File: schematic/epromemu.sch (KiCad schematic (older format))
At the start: 6 parts, among them J1 EPROM Connector, U1 Teensy4.1, U2 TXS0108EPW, U3 TXS0108EPW, U4 TXS0108EPW, U5 TXS0108EPW

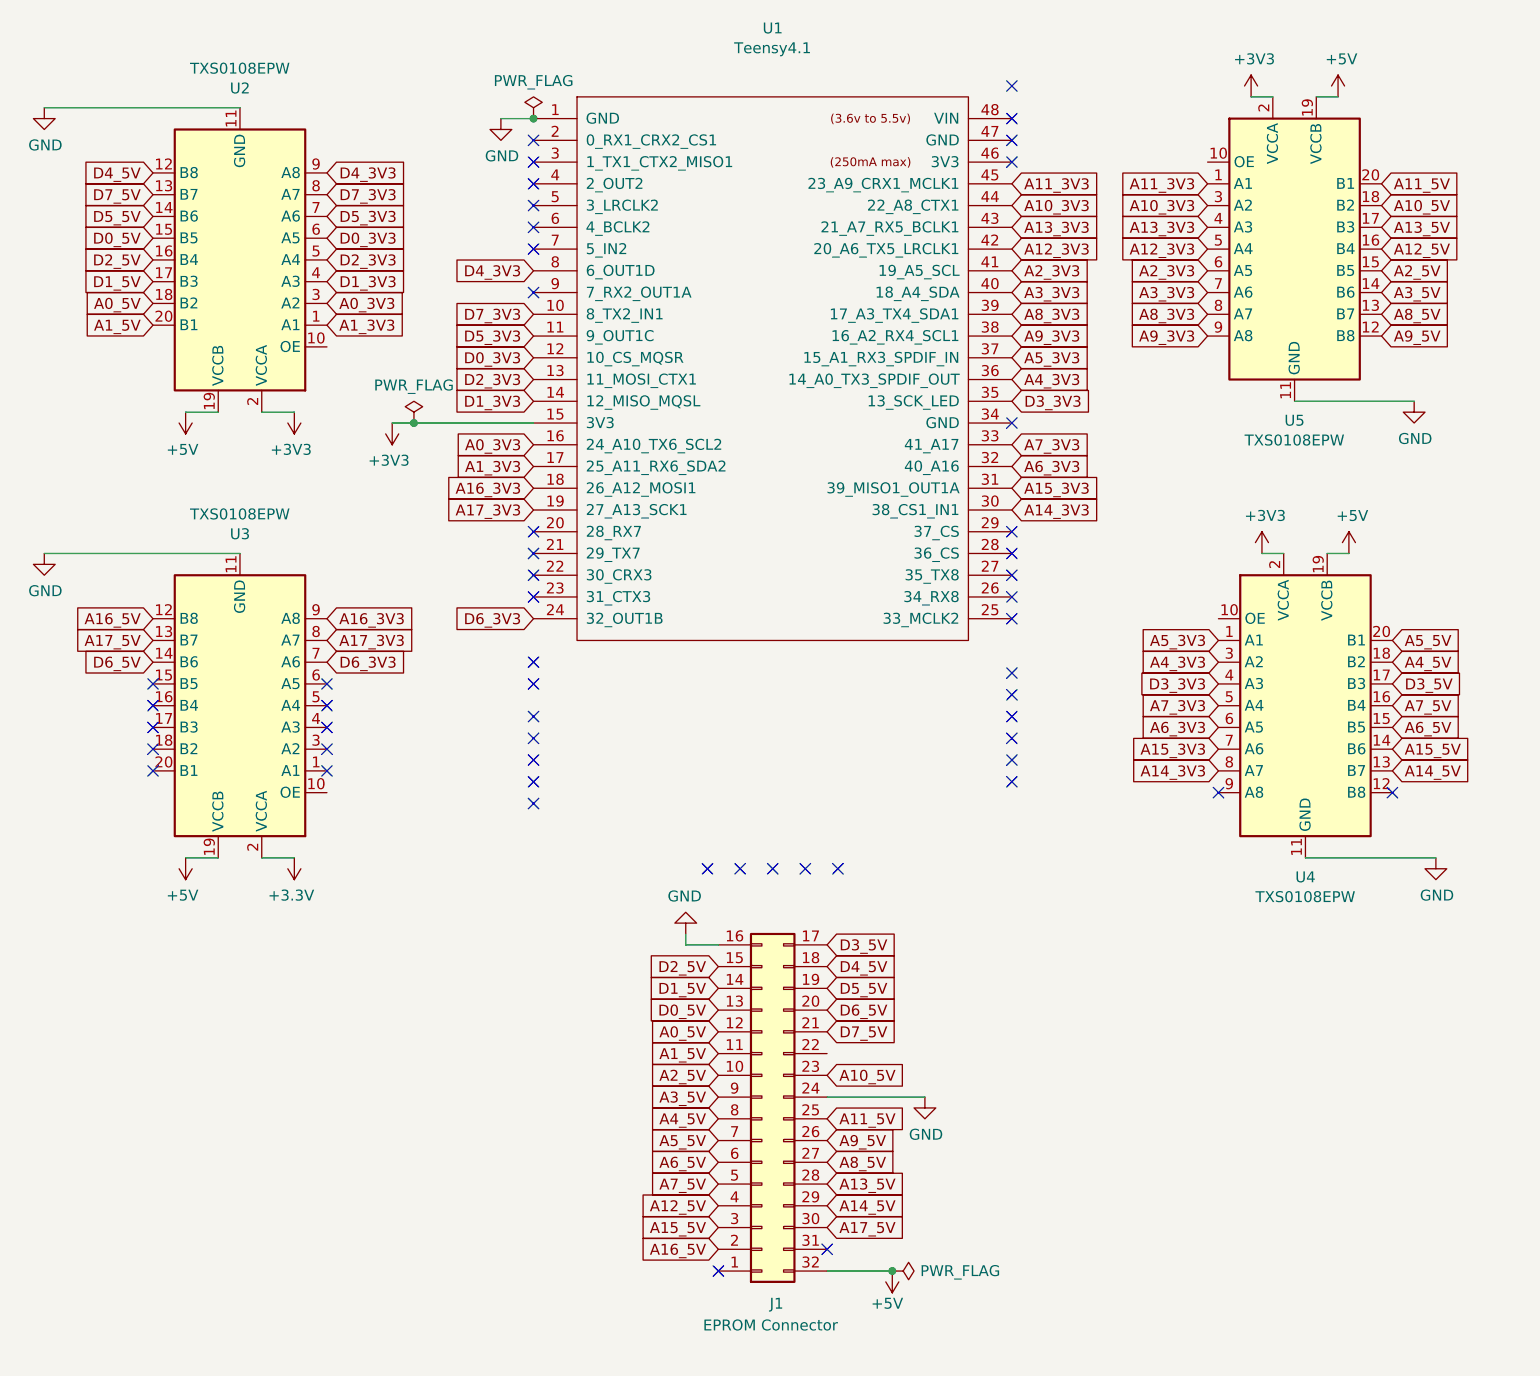
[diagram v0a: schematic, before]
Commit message: updates
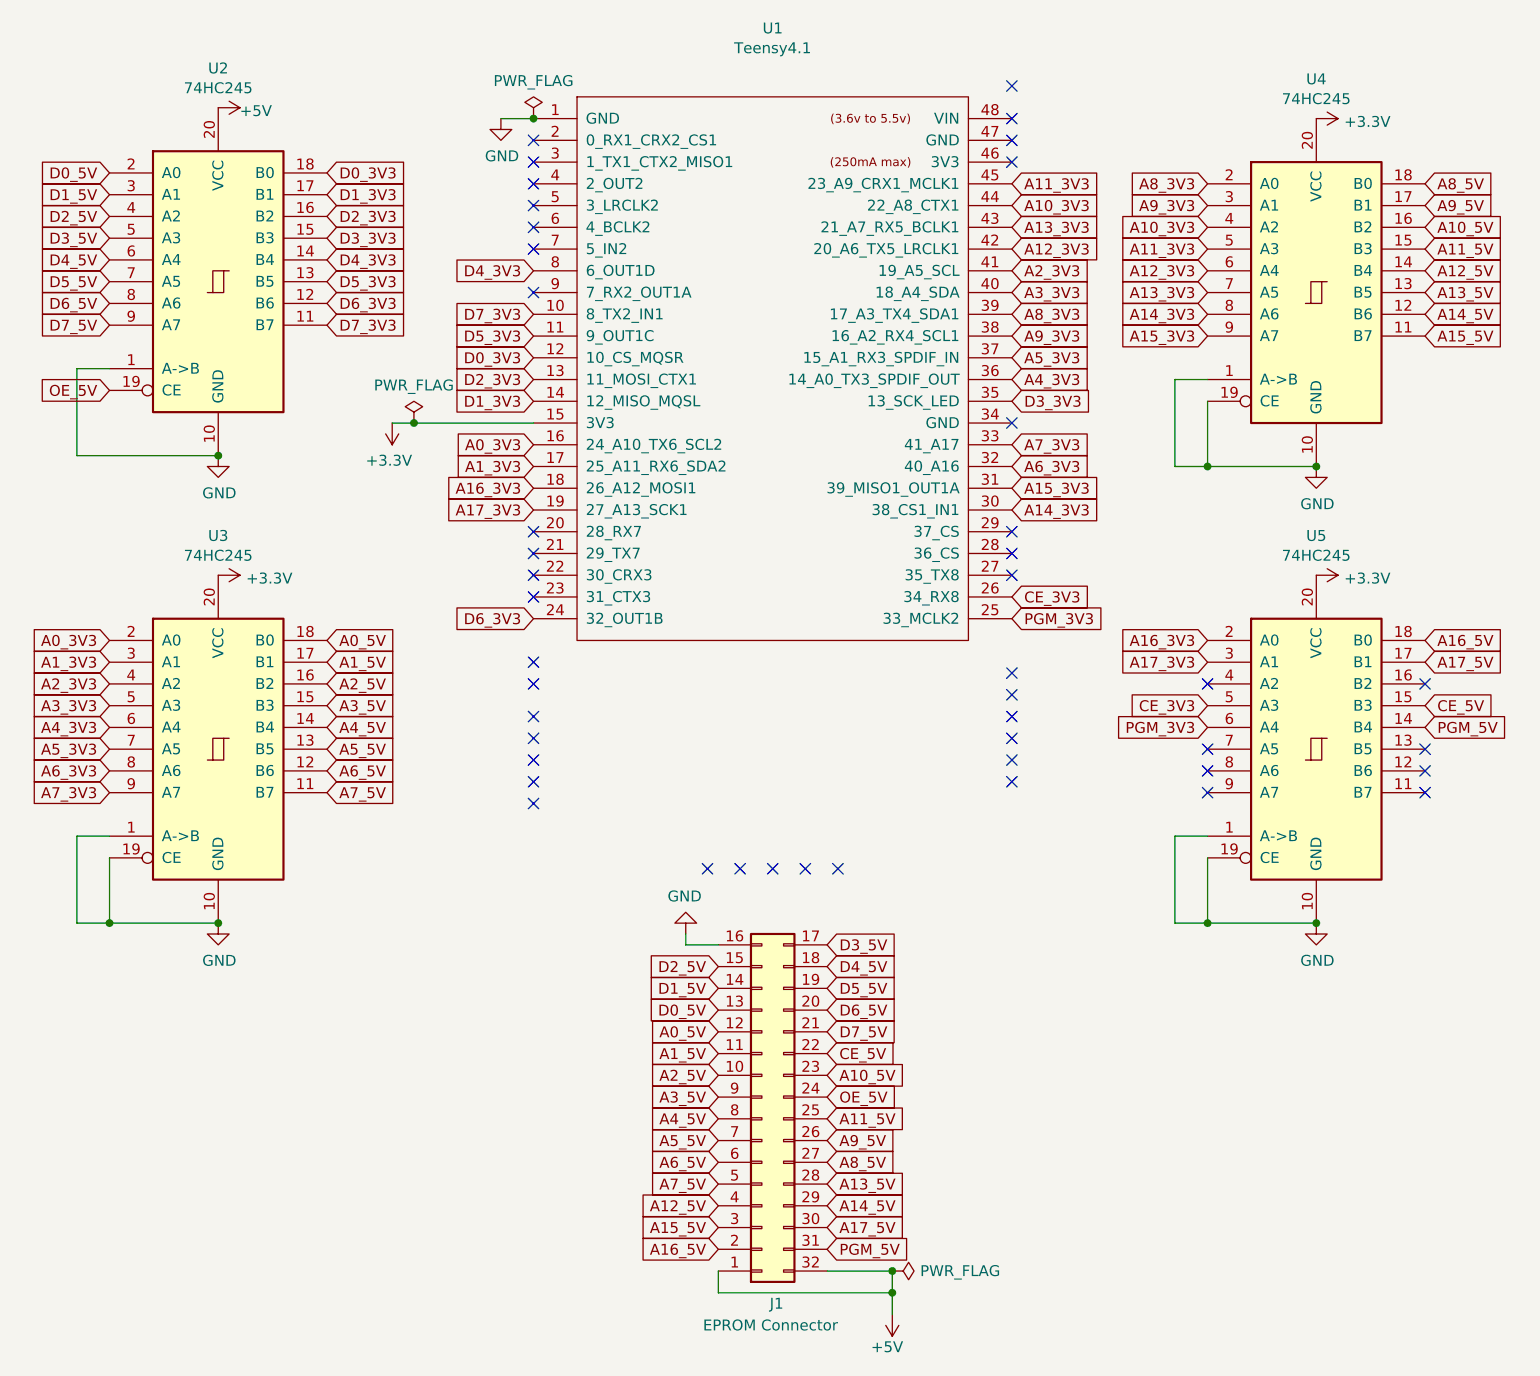
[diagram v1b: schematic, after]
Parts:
- removed U2, U3, U4, U5: TXS0108EPW, Package_SO:TSSOP-20_4.4x6.5mm_P0.65mm, symbol Logic_LevelTranslator:TXS0108EPW
- added U2, U3, U4, U5: 74HC245, Package_DIP:DIP-20_W7.62mm_Socket, symbol 74xx:74HC245
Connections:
- net +3V3: now also U3.20 (VCC), U4.20 (VCC), U5.20 (VCC)
- net +5V: now also J1.1 (Pin_1), U2.20 (VCC)
- net A0_3V3: now also U3.2 (A0)
- net A0_5V: now also U3.18 (B0)
- net A10_3V3: now also U4.4 (A2)
- net A10_5V: now also U4.16 (B2)
- net A11_3V3: now also U4.5 (A3)
- net A11_5V: now also U4.15 (B3)
- net A12_3V3: now also U4.6 (A4)
- net A12_5V: now also U4.14 (B4)
- net A13_3V3: now also U4.7 (A5)
- net A13_5V: now also U4.13 (B5)
- net A14_3V3: now also U4.8 (A6)
- net A14_5V: now also U4.12 (B6)
- net A15_3V3: now also U4.9 (A7)
- net A15_5V: now also U4.11 (B7)
- net A16_3V3: now also U5.2 (A0)
- net A16_5V: now also U5.18 (B0)
- net A17_3V3: now also U5.3 (A1)
- net A17_5V: now also U5.17 (B1)
- net A1_3V3: now also U3.3 (A1)
- net A1_5V: now also U3.17 (B1)
- net A2_3V3: now also U3.4 (A2)
- net A2_5V: now also U3.16 (B2)
- net A3_3V3: now also U3.5 (A3)
- net A3_5V: now also U3.15 (B3)
- net A4_3V3: now also U3.6 (A4)
- net A4_5V: now also U3.14 (B4)
- net A5_3V3: now also U3.7 (A5)
- net A5_5V: now also U3.13 (B5)
- net A6_3V3: now also U3.8 (A6)
- net A6_5V: now also U3.12 (B6)
- net A7_3V3: now also U3.9 (A7)
- net A7_5V: now also U3.11 (B7)
- net A8_3V3: now also U4.2 (A0)
- net A8_5V: now also U4.18 (B0)
- net A9_3V3: now also U4.3 (A1)
- net A9_5V: now also U4.17 (B1)
- net D0_3V3: now also U2.18 (B0)
- net D0_5V: now also U2.2 (A0)
- net D1_3V3: now also U2.17 (B1)
- net D1_5V: now also U2.3 (A1)
- net D2_3V3: now also U2.16 (B2)
- net D2_5V: now also U2.4 (A2)
- net D3_3V3: now also U2.15 (B3)
- net D3_5V: now also U2.5 (A3)
- net D4_3V3: now also U2.14 (B4)
- net D4_5V: now also U2.6 (A4)
- net D5_3V3: now also U2.13 (B5)
- net D5_5V: now also U2.7 (A5)
- net D6_3V3: now also U2.12 (B6)
- net D6_5V: now also U2.8 (A6)
- net D7_3V3: now also U2.11 (B7)
- net D7_5V: now also U2.9 (A7)
- net GND: now also U2.1 (A->B), U2.10 (GND), U3.1 (A->B), U3.10 (GND), U3.19 (CE), U4.1 (A->B), U4.10 (GND), U4.19 (CE), U5.1 (A->B), U5.10 (GND), U5.19 (CE); no longer J1.24 (Pin_24)
- net PGM_3V3: now reaches U1.25 (33_MCLK2)
- net PGM_3V3: now also U5.6 (A4)
- net CE_3V3: now reaches U1.26 (34_RX8)
- net CE_3V3: now also U5.5 (A3)
- net CE_5V: now reaches J1.22 (Pin_22)
- net CE_5V: now also U5.15 (B3)
- net PGM_5V: now reaches J1.31 (Pin_31)
- net PGM_5V: now also U5.14 (B4)
- new net OE_5V: J1.24 (Pin_24), U2.19 (CE)
- no-connect marks 53 -> 45
